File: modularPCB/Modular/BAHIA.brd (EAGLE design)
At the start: 100 x 80 mm, 3 parts

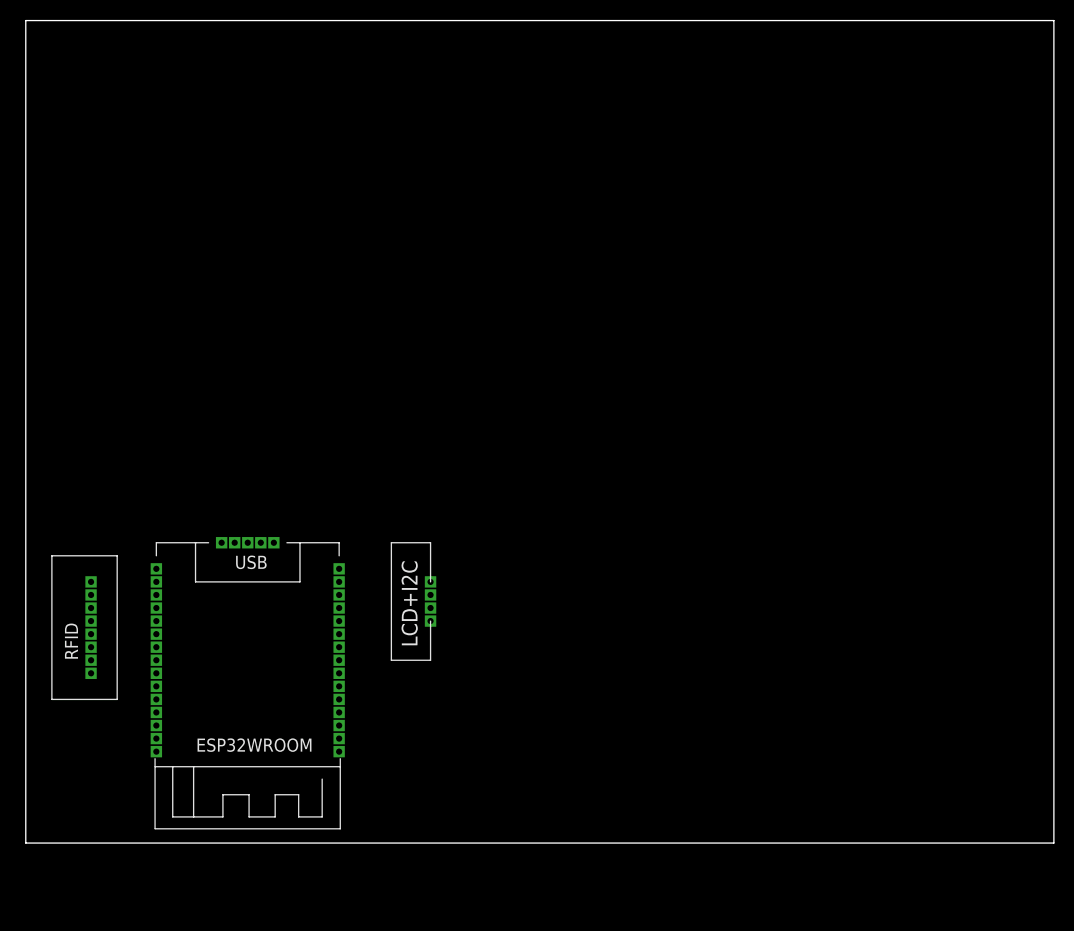
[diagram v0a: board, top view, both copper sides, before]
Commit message: Actualización de pcbs
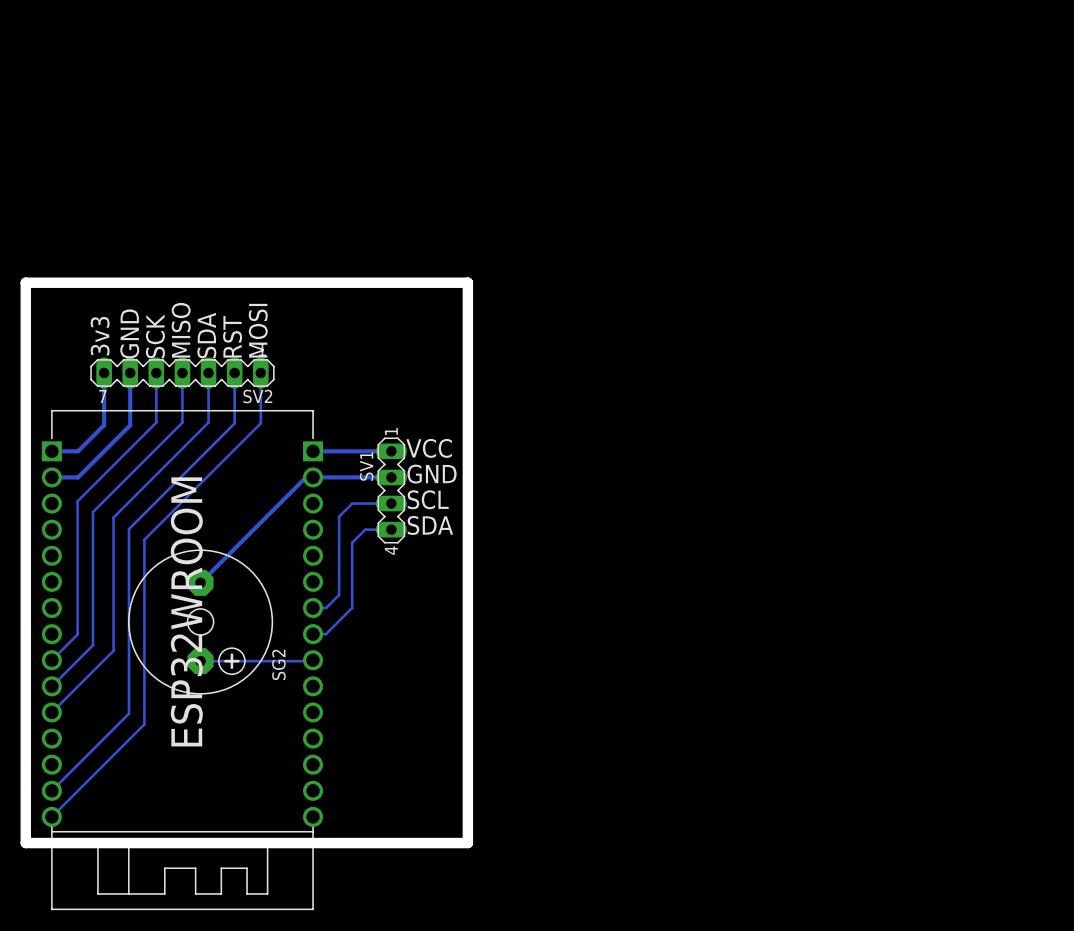
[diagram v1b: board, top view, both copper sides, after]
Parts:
- removed U$2: LCD+I2C, MODULAR:LCD
- removed U$3: RFID, MODULAR:RFID
- added SG2: F/CM12P, buzzer:F/CM12P
- added SV1: (no value), con-lstb:MA04-1
- added SV2: (no value), con-lstb:MA07-1
- moved U$1 25.9 mm to (27.9, 38.1), turned to 90 degrees
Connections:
- removed net N$1: U$1.D21, U$3.SDA
- removed net N$10: U$1.D26, U$2.SCL
- removed net N$11: U$1.D25, U$2.SDA
- removed net N$2: U$1.D18, U$3.SCK
- removed net N$3: U$1.D23, U$3.MOSI
- removed net N$4: U$1.D19, U$3.MISO
- removed net N$5: U$1.GND@1, U$3.GND
- removed net N$6: U$1.D22, U$3.RST
- removed net N$7: U$1.3V3, U$3.3.3V
- removed net N$8: U$1.VIN, U$2.VCC
- removed net N$9: U$1.GND@0, U$2.GND
- new net 3V3: SV2.7, U$1.3V3
- new net BUZZER: SG2.+, U$1.D33
- new net GND: SG2.-, SV1.2, SV2.6, U$1.GND@0, U$1.GND@1
- new net MISO: SV2.4, U$1.D19
- new net MOSI: SV2.1, U$1.D23
- new net RST: SV2.2, U$1.D22
- new net SCK: SV2.5, U$1.D18
- new net SCL: SV1.3, U$1.D26
- new net SDA: SV2.3, U$1.D21
- new net SDA_I2C: SV1.4, U$1.D25
- new net VCC: SV1.1, U$1.VIN
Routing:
- net MOSI: track 0.00 -> 51.6 mm
- net RST: track 0.00 -> 48.0 mm
- net SDA: track 0.00 -> 39.3 mm
- net GND: track 0.00 -> 37.6 mm
- net MISO: track 0.00 -> 35.7 mm
- net SCK: track 0.00 -> 32.1 mm
- net SCL: track 0.00 -> 16.3 mm
- net SDA_I2C: track 0.00 -> 15.5 mm
- net 3V3: track 0.00 -> 11.2 mm
- net BUZZER: track 0.00 -> 11.0 mm
- net VCC: track 0.00 -> 7.62 mm
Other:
- board size 100 x 80 mm -> 43 x 54.5 mm
- board text added: "3v3"
- board text added: "GND"
- board text added: "MISO"
- board text added: "MOSI"
- board text added: "RST"
- board text added: "SCK"
- board text added: "SCL"
- board text added: "SDA"
- board text added: "VCC"
